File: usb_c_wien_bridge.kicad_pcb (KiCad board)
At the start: 2 copper layers, 49 x 14 mm, 20 parts, among them J1 USB_C_Receptacle_USB2.0, J2 Conn_01x05_Female, U1 TL082

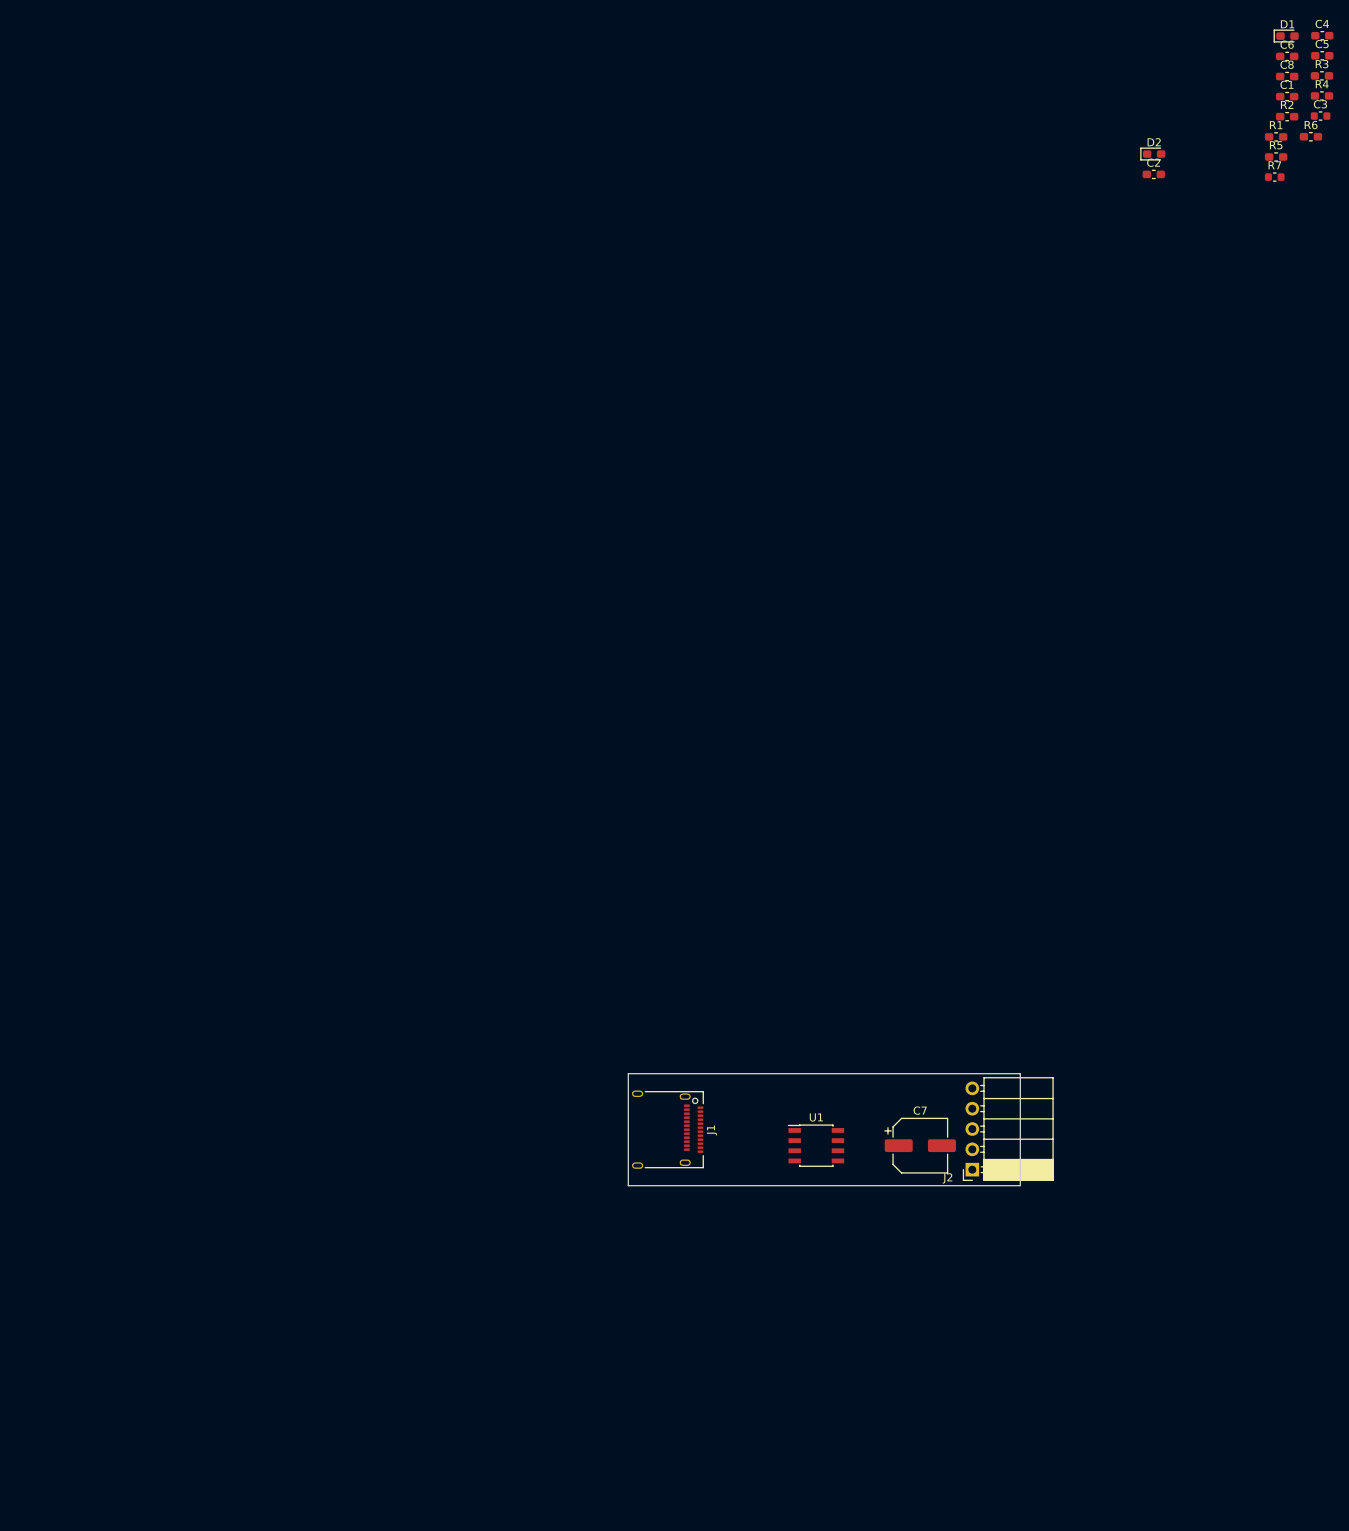
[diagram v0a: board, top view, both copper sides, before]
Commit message: Place all components. Needs routing.
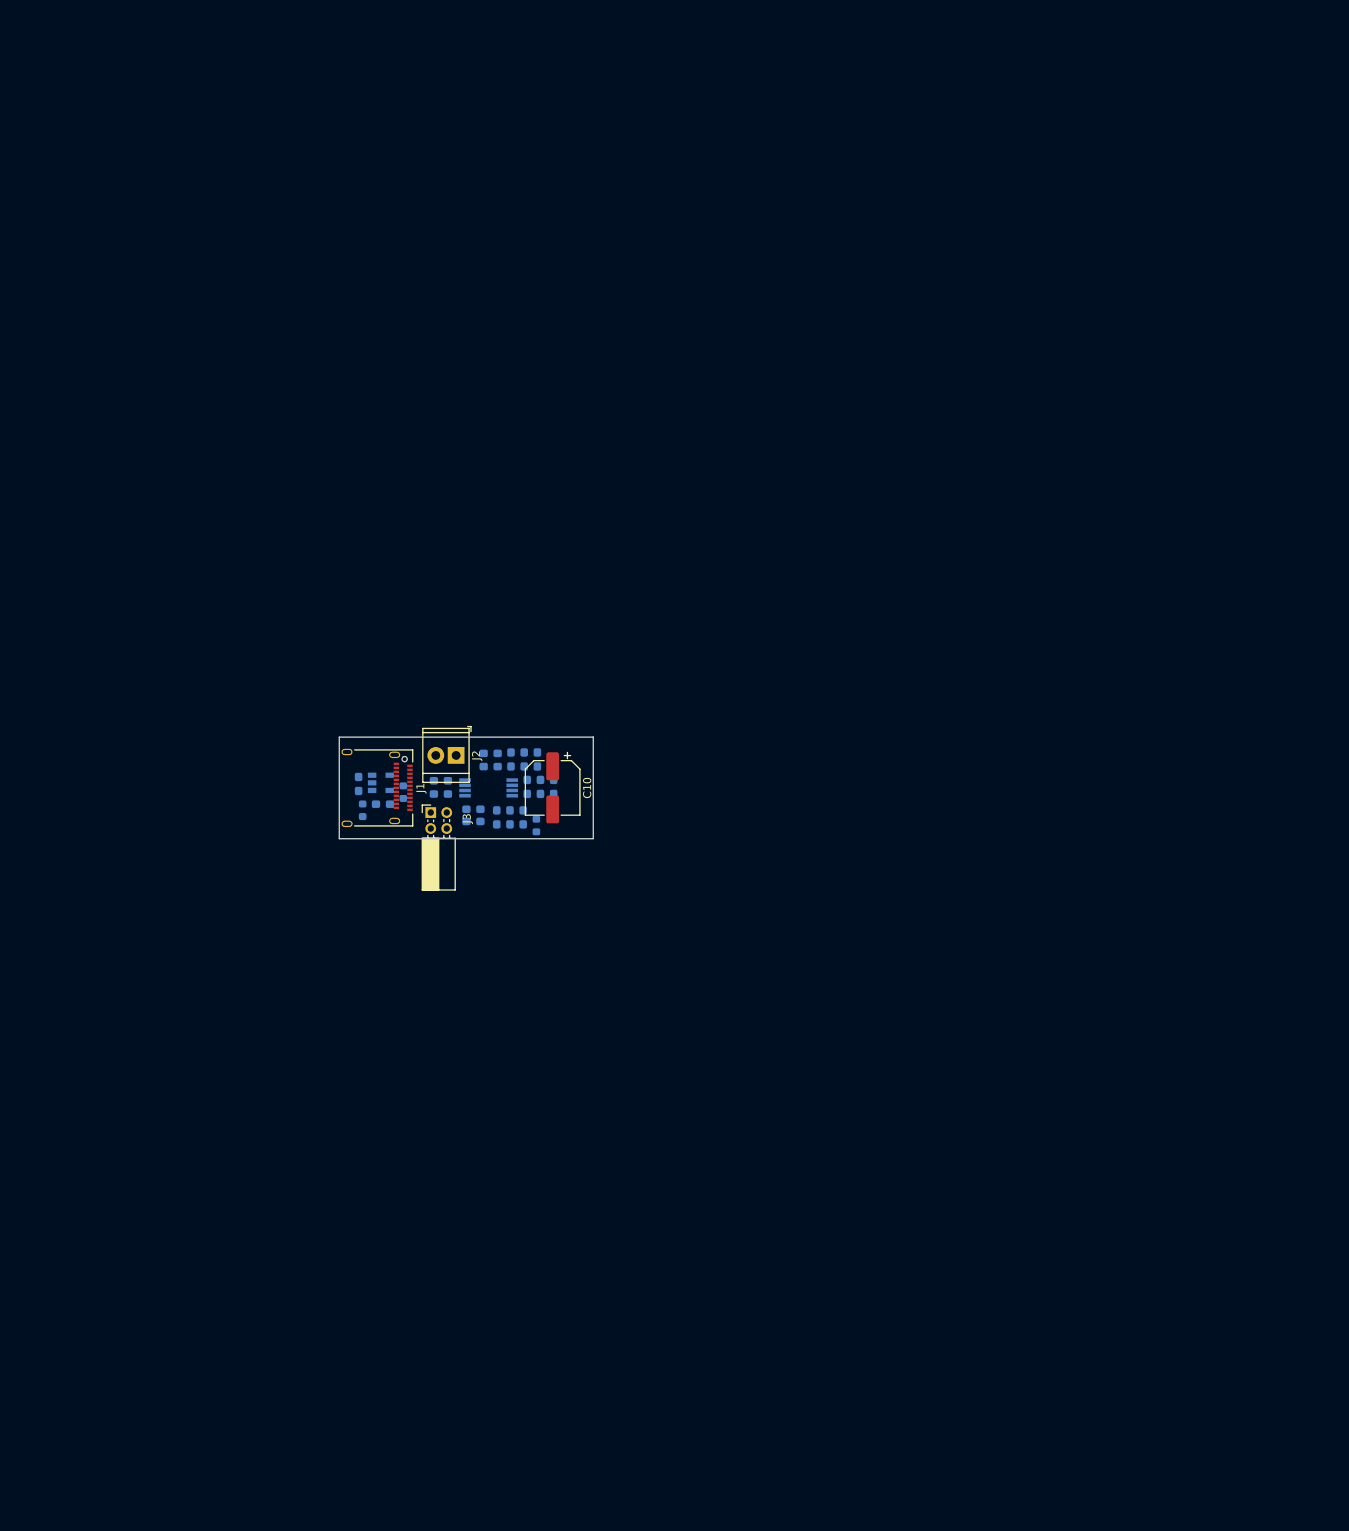
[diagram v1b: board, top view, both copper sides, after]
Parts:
- added C10: 47uF, Capacitor_SMD:CP_Elec_6.3x5.4_Nichicon, F.Cu at (193.0, 17.8)
- added C11: 1uF, Capacitor_SMD:C_0603_1608Metric_Pad1.05x0.95mm_HandSolder, B.Cu at (183.1, 22.0)
- added C12: 1uF, Capacitor_SMD:C_0603_1608Metric_Pad1.05x0.95mm_HandSolder, B.Cu at (183.1, 20.4)
- added C9: 1nF, Capacitor_SMD:C_0603_1608Metric_Pad1.05x0.95mm_HandSolder, B.Cu at (185.3, 13.5)
- added J3: Conn_02x02, Connector_PinSocket_2.00mm:PinSocket_2x02_P2.00mm_Horizontal, F.Cu at (177.8, 20.9)
- added U2: MIC5504-3.3YM5, Package_TO_SOT_SMD:SOT-23-5, B.Cu at (171.6, 17.1)
- C1, C2, D1, D2, R1, R2, R3, R4, R5, R6, R7: moved to B.Cu
- C3: value 0u1F -> 1uF; footprint Capacitor_SMD:C_0603_1608Metric -> Capacitor_SMD:C_0603_1608Metric_Pad1.05x0.95mm_HandSolder; moved to B.Cu
- C4: footprint Capacitor_SMD:C_0603_1608Metric_Pad1.05x0.95mm_HandSolder -> Capacitor_SMD:C_0603_1608Metric; moved to B.Cu
- C5: value 1nF -> 0u1F; moved to B.Cu
- C6: value 1nF -> 1uF; moved to B.Cu
- C7: value 47uF -> 0u1F; footprint Capacitor_SMD:CP_Elec_6.3x5.4_Nichicon -> Capacitor_SMD:C_0603_1608Metric; moved to B.Cu
- C8: value 1uF -> 1nF; moved to B.Cu
- J1: footprint Connector_USB:USB_C_Receptacle_Amphenol_12401610E4-2A -> Amphenol:USB_C_Receptacle_Amphenol_12401610E4-2A
- J2: value Conn_01x05_Female -> Screw_Terminal_01x02; footprint Connector_PinSocket_2.54mm:PinSocket_1x05_P2.54mm_Horizontal -> TerminalBlock_TE-Connectivity:TerminalBlock_TE_282834-2_1x02_P2.54mm_Horizontal
- U1: value TL082 -> LMV358; footprint Package_SO:SOIC-8_3.9x4.9mm_P1.27mm -> Package_SO:TSSOP-8_4.4x3mm_P0.65mm; moved to B.Cu
- moved C4 154.2 mm to (169.3, 20.6), turned to 270 degrees
- moved C6 146.7 mm to (171.8, 19.8), turned to 180 degrees
- moved C5 140.4 mm to (186.1, 21.5), turned to 270 degrees
- moved R2 134.5 mm to (179.1, 16.9), turned to 180 degrees
- moved C3 134.0 mm to (187.7, 21.5), turned to 270 degrees
- moved R4 133.5 mm to (185.3, 15.1), turned to 180 degrees
- moved R1 132.8 mm to (179.1, 18.5)
- moved C1 131.3 mm to (189.4, 21.5), turned to 270 degrees
- moved D1 131.2 mm to (193.2, 17.7), turned to 270 degrees
- moved R3 130.1 mm to (191.1, 14.2), turned to 90 degrees
- moved C8 129.2 mm to (187.8, 14.2), turned to 270 degrees
- moved R6 125.4 mm to (189.5, 14.2), turned to 90 degrees
- moved C2 125.2 mm to (168.8, 17.3), turned to 90 degrees
- moved R7 122.8 mm to (191.0, 22.5), turned to 270 degrees
- moved R5 122.3 mm to (189.9, 17.7), turned to 90 degrees
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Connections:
- net Net-(D1-Pad1) renamed /NEG_FB
- C1 pad 1: +5V0 -> +3V3
- C3 pad 1: +5V0 -> +3V3
- C4 pad 1: Net-(C4-Pad1) -> +5V0
- C5 pad 1: Net-(C5-Pad1) -> /V_DIV
- C5 pad 2: Net-(C5-Pad2) -> GNDA
- C6 pad 1: /RAIL_SPLIT -> +3V3
- C6 pad 2: Net-(C5-Pad2) -> GNDA
- C7 pad 1: Net-(C7-Pad1) -> +3V3
- C7 pad 2: Net-(C7-Pad2) -> GNDA
- C8 pad 1: +5V0 -> Net-(C8-Pad1)
- C8 pad 2: GNDA -> /POS_FB
- D1 pad 2: Net-(C7-Pad1) -> Net-(C10-Pad1)
- D2 pad 1: Net-(C7-Pad1) -> Net-(C10-Pad1)
- J1 pad A5: (no net) -> Net-(J1-PadA5)
- J1 pad A6: (no net) -> Net-(J1-PadA6)
- J1 pad A7: (no net) -> Net-(J1-PadA7)
- J1 pad A8: (no net) -> Net-(J1-PadA8)
- J1 pad B5: (no net) -> Net-(J1-PadB5)
- J1 pad B6: (no net) -> Net-(J1-PadB6)
- J1 pad B7: (no net) -> Net-(J1-PadB7)
- J1 pad B8: (no net) -> Net-(J1-PadB8)
- J2 pad 1: GNDA -> Net-(J2-Pad1)
- J2 pad 2: Net-(C7-Pad2) -> +5V0
- R1 pad 1: +5V0 -> +3V3
- R1 pad 2: Net-(C4-Pad1) -> /V_DIV
- R2 pad 1: Net-(C4-Pad1) -> /V_DIV
- R4 pad 1: Net-(C5-Pad2) -> /POS_FB
- R5 pad 1: Net-(C7-Pad1) -> Net-(C10-Pad1)
- R6 pad 1: Net-(C7-Pad1) -> Net-(C10-Pad1)
- R6 pad 2: Net-(C5-Pad1) -> Net-(C8-Pad1)
- R7 pad 1: Net-(C7-Pad2) -> /A_OUT
- U1 pad 2: Net-(C4-Pad1) -> /RAIL_SPLIT
- U1 pad 3: GNDA -> /V_DIV
- U1 pad 5: Net-(C5-Pad2) -> /POS_FB
- U1 pad 7: Net-(C7-Pad1) -> Net-(C10-Pad1)
- U1 pad 8: +5V0 -> +3V3
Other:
- board size 49 x 14 mm -> 31.8 x 12.7 mm

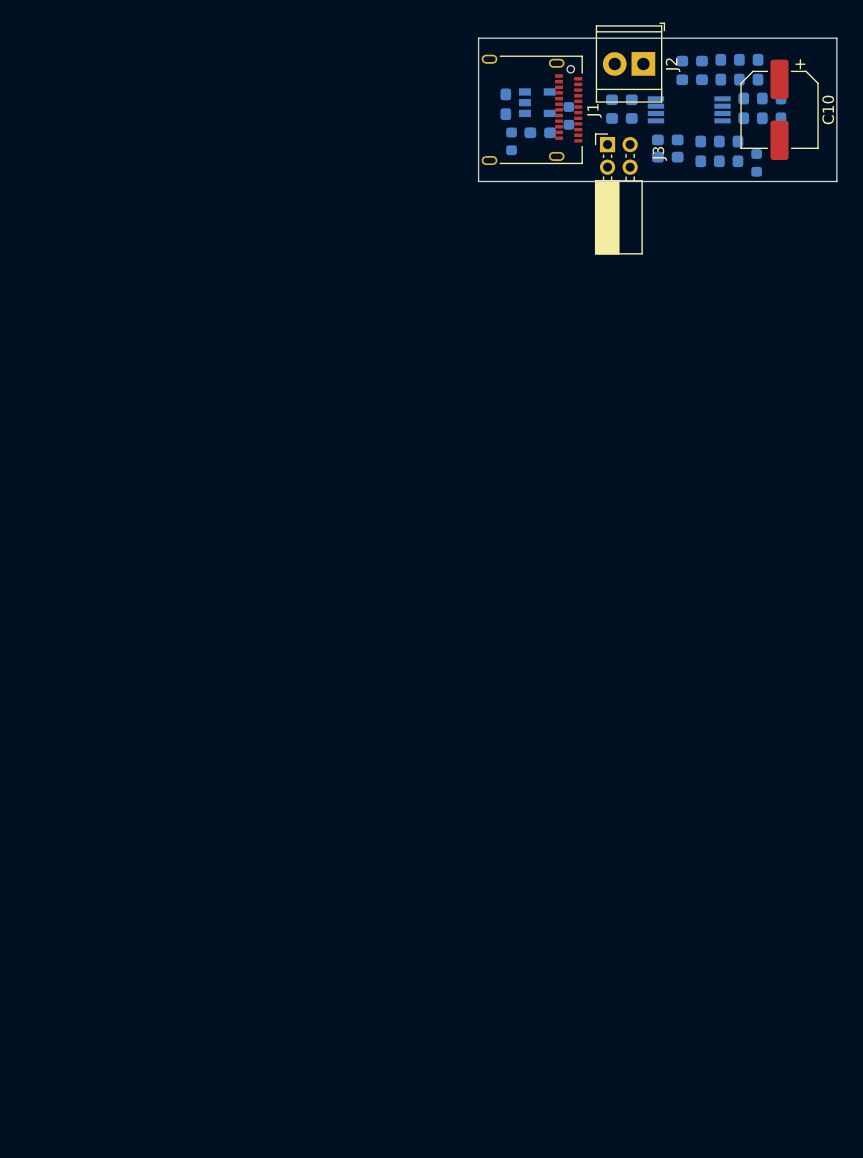
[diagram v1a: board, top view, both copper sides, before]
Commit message: Finish routing
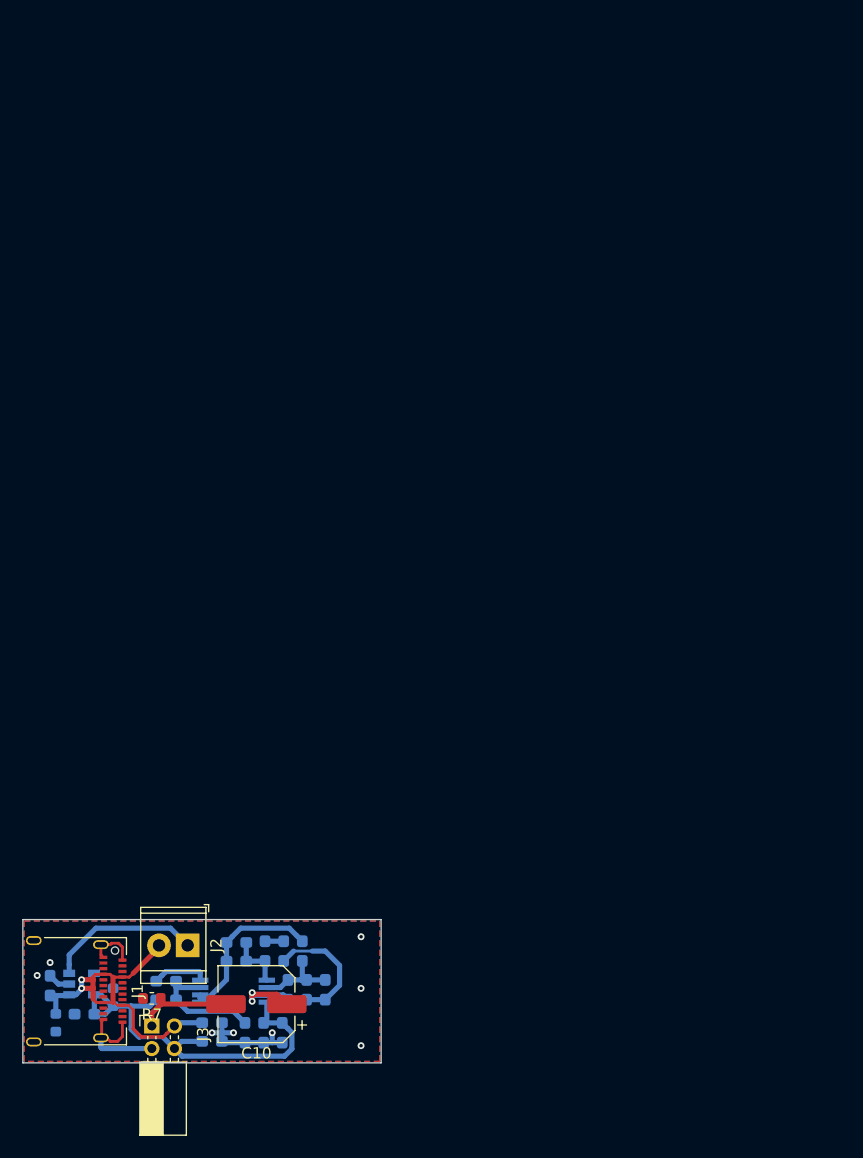
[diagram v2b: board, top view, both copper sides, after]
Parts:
- R7: moved to F.Cu
- moved C10 91.8 mm to (146.7, 97.0), turned to 180 degrees
- moved R7 91.4 mm to (137.4, 96.5), turned to 180 degrees
- moved C12 89.5 mm to (142.7, 100.3)
- moved J3 87.9 mm to (137.4, 99.0)
- moved C2 87.9 mm to (128.4, 95.4)
- moved C4 87.9 mm to (128.9, 98.7)
- moved C6 87.9 mm to (131.4, 97.9)
- moved J1 87.9 mm to (129.8, 95.9)
- moved J2 87.9 mm to (140.6, 91.8)
- moved R1 87.9 mm to (138.7, 96.6)
- moved R4 87.9 mm to (144.9, 93.2)
- moved U1 87.9 mm to (144.7, 95.9)
- moved U2 87.9 mm to (131.2, 95.2)
- moved C1 87.9 mm to (149.0, 99.6)
- moved C3 87.9 mm to (147.3, 99.6)
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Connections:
- J3 pad 1: GNDA -> /A_OUT
- J3 pad 2: /A_OUT -> GNDA
- J3 pad 3: +3V3 -> +5V0
- J3 pad 4: +5V0 -> +3V3
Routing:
- net +3V3: track 0.00 -> 36.0 mm
- net GNDA: track 0.00 -> 31.9 mm, vias 0 -> 8
- net +5V0: track 0.00 -> 31.6 mm, vias 0 -> 2
- net Net-(C10-Pad1): track 0.00 -> 22.2 mm, vias 0 -> 2
- net /RAIL_SPLIT: track 0.00 -> 14.7 mm
- net Net-(J2-Pad1): track 0.00 -> 13.7 mm
- net /V_DIV: track 0.00 -> 10.8 mm
- net /A_OUT: track 0.00 -> 8.55 mm
- net /NEG_FB: track 0.00 -> 7.18 mm
- net /POS_FB: track 0.00 -> 5.09 mm
- net Net-(C8-Pad1): track 0.00 -> 1.65 mm
- added copper zone on B.Cu, net GNDA
- added copper zone on F.Cu, net GNDA
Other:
- net class OSH Park Minimums added: clearance 0.1524, trace_width 0.1524, via_dia 0.508, via_drill 0.254
- rule pad_to_mask_clearance: 0.051 -> 0.0508
- rule solder_mask_min_width: 0.25 -> 0.1016
- rule trace_min: 0.2 -> 0.1524
- rule via_min_drill: 0.3 -> 0.254
- rule via_min_size: 0.4 -> 0.508
